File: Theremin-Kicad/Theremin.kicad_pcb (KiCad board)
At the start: 2 copper layers, 131.8 x 80 mm, 36 parts, among them CON1 BARREL_JACK, P1 SENSOR_1_NOTA, P2 SENSOR_2_VOL, P3 FPGA_OUTS, P4 FPGA_INS, P5 AUDIO_OUT, P6 CONN_2, SW1 VOL_UP, SW2 VOL_DOWN, SW3 PITCH_UP, SW4 PITCH_DOWN, SW5 MODE, SW6 SET, U1 NCP1117ST33T3G, U2 LM78M05CT, U3 X9C104P

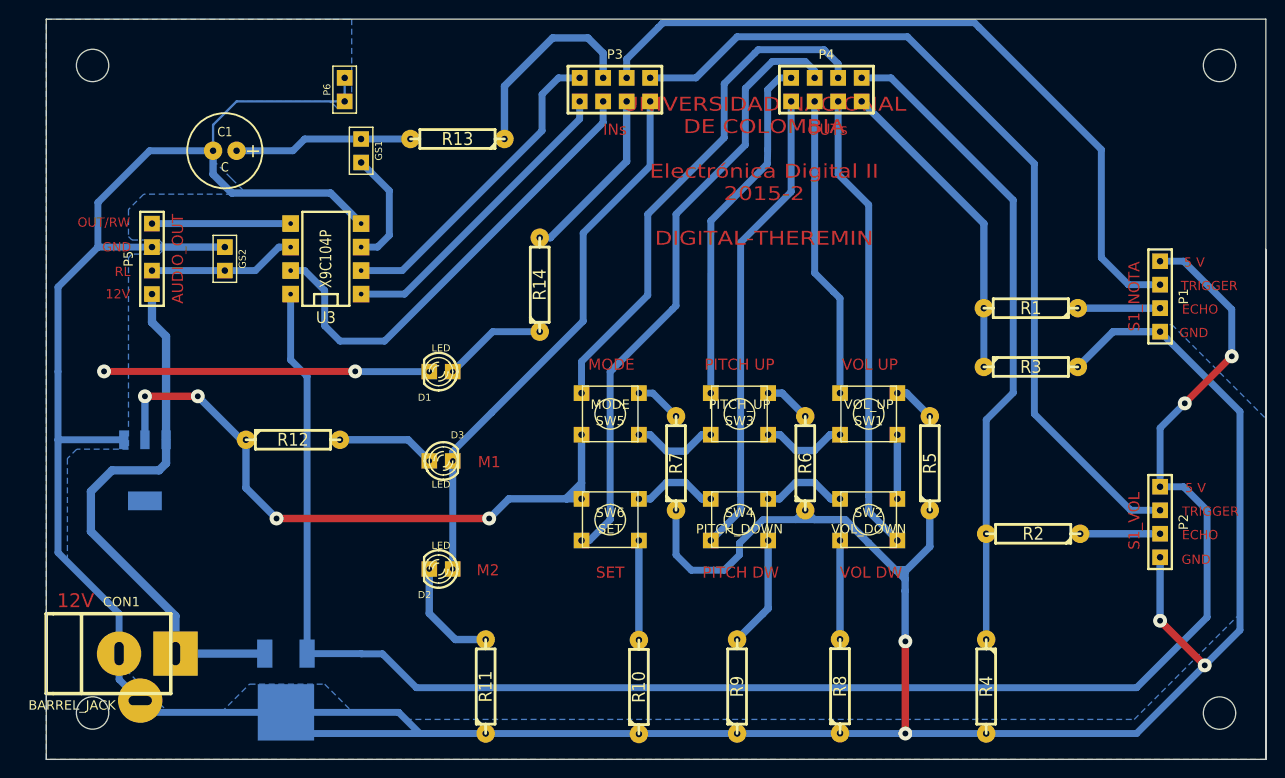
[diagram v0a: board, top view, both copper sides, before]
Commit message: 27Nov-PCB&PWM
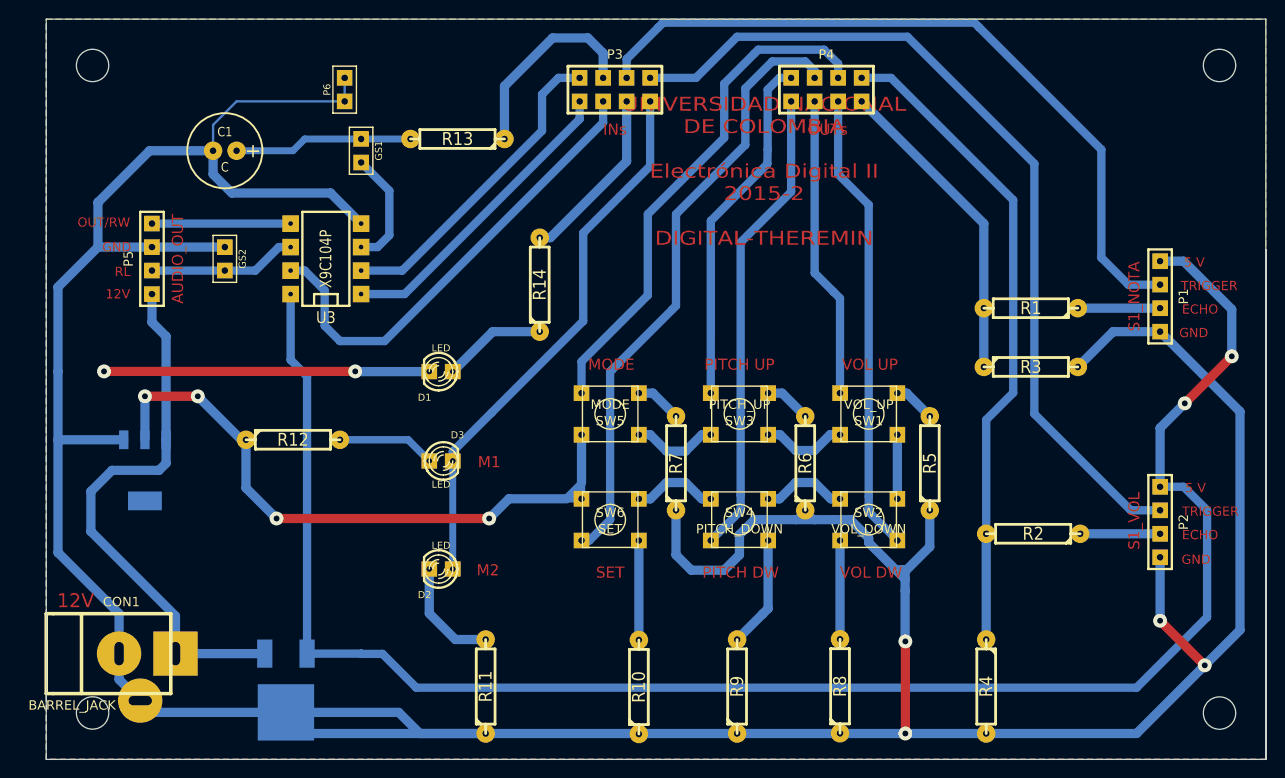
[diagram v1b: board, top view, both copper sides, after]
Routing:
- net GND: track 444.2 -> 445.1 mm
- added copper zone on F.Cu, net (none)
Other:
- net class 1 removed
- net class 2 removed
- net class 3 removed
- net class 4 removed
- net class 5 removed
- net class 6 removed
- net class NWO added: clearance 0.3, trace_width 1, via_dia 1.5, via_drill 0.6
